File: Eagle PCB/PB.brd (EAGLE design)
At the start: 43.6 x 39.1 mm, 25 parts, among them IC1 74HC595D, IC2 74HC595D, IC3 L78LXXCU/BU, J1 61300511121, J2 61300211121, J3 61300211121, J4 61300511121, J5 61300211121, J6 61300511121, J7 61300211121

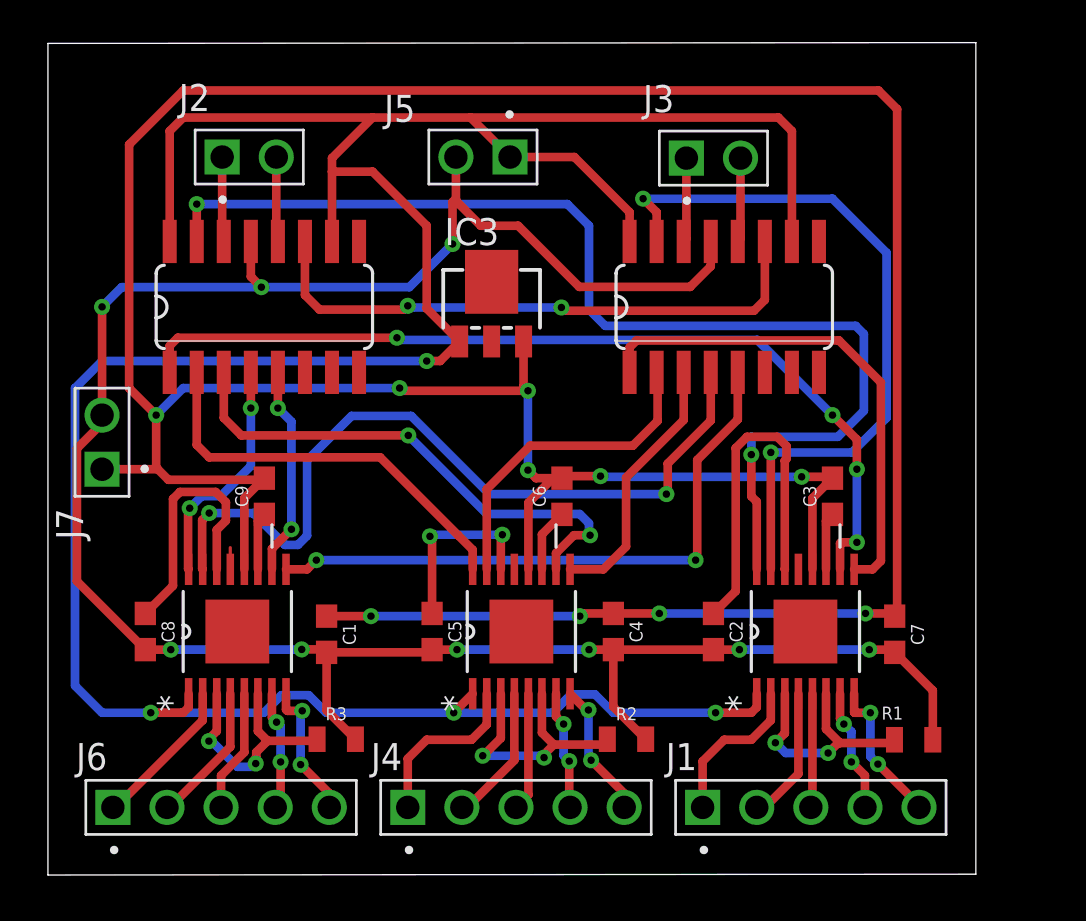
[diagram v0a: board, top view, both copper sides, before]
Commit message: Final PCB schematic and board added.
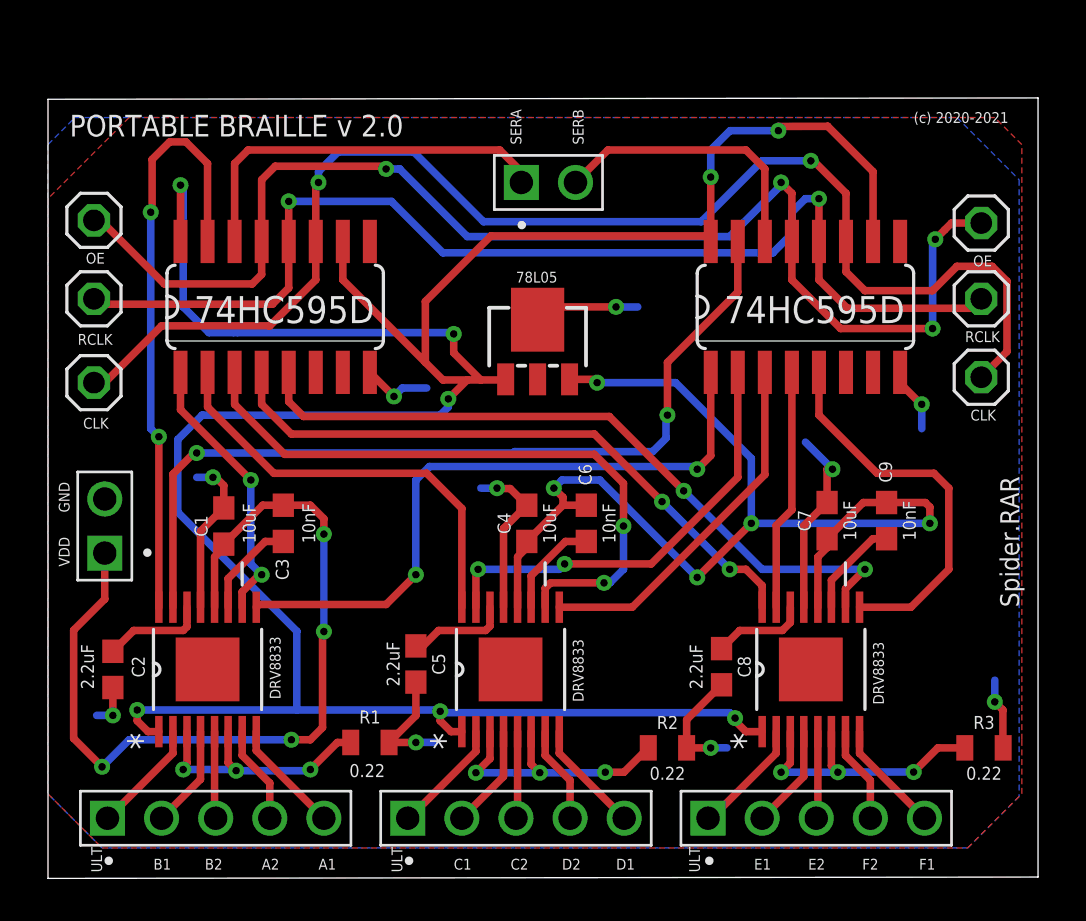
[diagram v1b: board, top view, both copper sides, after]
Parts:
- removed J3, J5: 61300211121, Headers:61300211121
- added JP1, JP2, JP3, JP4, JP5, JP6: (no value), pinhead:1X01
- moved R3 30.4 mm to (43.9, 5.97)
- moved C9 29.2 mm to (39.4, 16.6)
- moved C2 28.3 mm to (3.05, 9.65)
- moved DRV8833PWP1 28.1 mm to (7.49, 9.65)
- moved J1 27.9 mm to (7.87, 2.67)
- moved J6 27.9 mm to (36.1, 2.67)
- moved C8 27.1 mm to (31.6, 9.78)
- moved DRV8833PWP3 27.0 mm to (35.8, 9.65)
- moved C3 25.8 mm to (11.0, 16.5)
- moved R1 25.5 mm to (15.1, 6.22)
- moved J2 14.1 mm to (23.5, 32.5)
- moved C1 7.01 mm to (8.26, 16.4), turned to 90 degrees
- moved C4 6.51 mm to (22.5, 16.5), turned to 90 degrees
- moved C7 6.21 mm to (36.6, 16.6), turned to 90 degrees
- moved J7 3.94 mm to (2.67, 16.4)
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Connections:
- net N$11 renamed SA
- removed net GND: IC1.8, IC2.8, IC3.4
- removed net N$1: IC1.12, J2.2
- removed net N$12: IC2.14, J3.1
- removed net N$25: IC2.12, J3.2
- new net OE: IC1.13, IC2.13, JP1.1, JP4.1
- new net RCK: IC1.12, IC2.12, JP2.1, JP5.1
- new net SB: IC2.14, J2.2
- net 0: now also IC1.8, IC2.8, IC3.4; no longer IC1.13, IC2.13, J5.2
- net CLK: now also JP3.1, JP6.1
- net VCC: no longer J5.1
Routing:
- net VDD: track 165.0 -> 92.5 mm, vias 10 -> 9
- net OE: track 0.00 -> 60.0 mm, vias 0 -> 4
- net 0: track 108.1 -> 52.1 mm, vias 9 -> 10
- net RCK: track 0.00 -> 53.3 mm, vias 0 -> 2
- net CLK: track 27.5 -> 63.3 mm
- net B1: track 42.7 -> 13.0 mm, vias 4 -> 2
- net E2: track 37.6 -> 11.3 mm, vias 2 -> 0
- net A1: track 53.6 -> 28.3 mm
- net F1: track 9.89 -> 33.8 mm
- net E1: track 11.0 -> 29.5 mm
- net SA: track 3.99 -> 18.3 mm
- net SB: track 0.00 -> 13.3 mm
- net N$2: track 16.8 -> 4.87 mm
- net F2: track 29.1 -> 18.3 mm, vias 2 -> 0
- net N$21: track 12.1 -> 4.45 mm
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- added copper zone on layer 16, net 0
- added copper zone on layer 1, net VDD
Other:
- board size 43.6 x 39.1 mm -> 46.5 x 36.6 mm
- board text added: "(c) 2020-2021"
- board text added: "78L05"
- board text added: "A1"
- board text added: "A2"
- board text added: "B1"
- board text added: "B2"
- board text added: "C1"
- board text added: "C2"
- board text added: "CLK"
- board text added: "D1"
- board text added: "D2"
- board text added: "DRV8833"
- board text added: "E1"
- board text added: "E2"
- board text added: "F1"
- board text added: "F2"
- board text added: "GND"
- board text added: "OE"
- board text added: "PORTABLE BRAILLE v 2.0"
- board text added: "RCLK"
- board text added: "SERA"
- board text added: "SERB"
- board text added: "Spider.RAR"
- board text added: "ULT"
- board text added: "VDD"
